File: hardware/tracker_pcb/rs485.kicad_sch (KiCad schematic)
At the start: 5 parts, among them IC3 THVD1426DRLR

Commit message: add opto input module
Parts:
- IC3: footprint SOTFL50P160X60-8N -> footprint:SOTFL50P160X60-8N
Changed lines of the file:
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@@
 			)
 		)
-		(property "Footprint" "SOTFL50P160X60-8N"
+		(property "Footprint" "footprint:SOTFL50P160X60-8N"
 			(at 144.78 169.85 0)
 			(effects

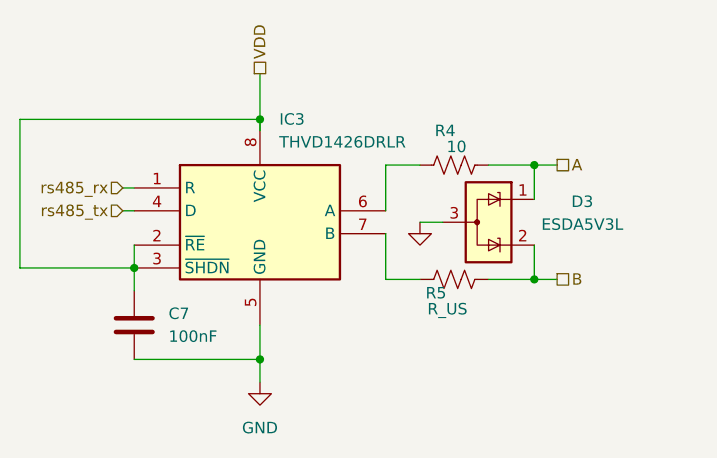
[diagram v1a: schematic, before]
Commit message: Work
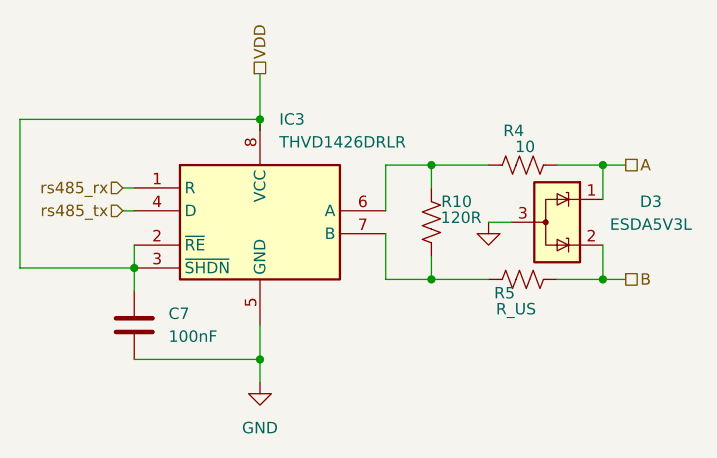
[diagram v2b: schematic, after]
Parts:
- added R10: 120R, Resistor_SMD:R_0603_1608Metric, symbol Device:R_US
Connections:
- net at IC3.6 (A), R4.1: now also R10.2
- net at IC3.7 (B), R5.1: now also R10.1
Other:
- moved on the sheet: D3, R4, R5
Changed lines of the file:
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@@
 	)
 	(junction
-		(at 165.1 72.39)
+		(at 172.72 72.39)
 		(diameter 0)
 		(color 0 0 0 0)
 	)
 	(junction
-		(at 165.1 85.09)
+		(at 172.72 85.09)
+		(diameter 0)
+		(color 0 0 0 0)
+	)
+	(junction
+		(at 153.67 72.39)
 		(diameter 0)
 		(color 0 0 0 0)
@@
 	)
 	(junction
+		(at 153.67 85.09)
+		(diameter 0)
+		(color 0 0 0 0)
+	)
+	(junction
 		(at 134.62 67.31)
 		(diameter 0)
@@
 	(wire
 		(pts
-			(xy 160.02 85.09) (xy 165.1 85.09)
+			(xy 167.64 85.09) (xy 172.72 85.09)
 		)
 		(stroke
@@
 	(wire
 		(pts
+			(xy 153.67 72.39) (xy 153.67 74.93)
+		)
+		(stroke
+			(width 0)
+			(type default)
+		)
+	)
+	(wire
+		(pts
 			(xy 134.62 93.98) (xy 134.62 96.52)
 		)
@@
 	(wire
 		(pts
-			(xy 165.1 72.39) (xy 165.1 76.2)
+			(xy 172.72 72.39) (xy 172.72 76.2)
 		)
 		(stroke
@@
 	(wire
 		(pts
-			(xy 160.02 72.39) (xy 165.1 72.39)
+			(xy 167.64 72.39) (xy 172.72 72.39)
+		)
+		(stroke
+			(width 0)
+			(type default)
+		)
+	)
+	(wire
+		(pts
+			(xy 153.67 72.39) (xy 160.02 72.39)
 		)
 		(stroke
@@
 	(wire
 		(pts
-			(xy 165.1 85.09) (xy 167.64 85.09)
+			(xy 153.67 82.55) (xy 153.67 85.09)
+		)
+		(stroke
+			(width 0)
+			(type default)
+		)
+	)
+	(wire
+		(pts
+			(xy 172.72 85.09) (xy 175.26 85.09)
 		)
 		(stroke
@@
 	(wire
 		(pts
+			(xy 153.67 85.09) (xy 160.02 85.09)
+		)
+		(stroke
+			(width 0)
+			(type default)
+		)
+	)
+	(wire
+		(pts
 			(xy 120.65 83.82) (xy 120.65 86.36)
 		)
@@
 	(wire
 		(pts
-			(xy 165.1 72.39) (xy 167.64 72.39)
-		)
-		(stroke
-			(width 0)
-			(type default)
-		)
-	)
-	(wire
-		(pts
-			(xy 152.4 78.74) (xy 154.94 78.74)
+			(xy 172.72 72.39) (xy 175.26 72.39)
+		)
+		(stroke
+			(width 0)
+			(type default)
+		)
+	)
+	(wire
+		(pts
+			(xy 160.02 78.74) (xy 162.56 78.74)
 		)
 		(stroke
@@
 	(wire
 		(pts
-			(xy 165.1 85.09) (xy 165.1 81.28)
+			(xy 172.72 85.09) (xy 172.72 81.28)
 		)
 		(stroke
@@
 	(wire
 		(pts
-			(xy 148.59 72.39) (xy 152.4 72.39)
-		)
-		(stroke
-			(width 0)
-			(type default)
-		)
-	)
-	(wire
-		(pts
-			(xy 148.59 85.09) (xy 152.4 85.09)
+			(xy 148.59 72.39) (xy 153.67 72.39)
+		)
+		(stroke
+			(width 0)
+			(type default)
+		)
+	)
+	(wire
+		(pts
+			(xy 148.59 85.09) (xy 153.67 85.09)
 		)
 		(stroke
@@
 	(hierarchical_label "B"
 		(shape passive)
-		(at 167.64 85.09 0)
+		(at 175.26 85.09 0)
 		(effects
 			(font
@@
 	(hierarchical_label "A"
 		(shape passive)
-		(at 167.64 72.39 0)
+		(at 175.26 72.39 0)
 		(effects
 			(font
@@
 	(symbol
 		(lib_id "Power_Protection:ESDA5V3L")
-		(at 160.02 78.74 270)
+		(at 167.64 78.74 270)
 		(unit 1)
 		(exclude_from_sim no)
@@
 		(dnp no)
 		(property "Reference" "D3"
-			(at 170.434 76.454 90)
+			(at 178.054 76.454 90)
 			(effects
 				(font
@@
 		)
 		(property "Value" "ESDA5V3L"
-			(at 170.434 78.994 90)
+			(at 178.054 78.994 90)
 			(effects
 				(font
@@
 		)
 		(property "Footprint" "Package_TO_SOT_SMD:SOT-23-3"
-			(at 149.86 63.5 0)
+			(at 157.48 63.5 0)
 			(effects
 				(font
@@
 		)
 		(property "Datasheet" "https://www.st.com/resource/en/datasheet/esdal.pdf"
-			(at 144.78 78.74 0)
+			(at 152.4 78.74 0)
 			(effects
 				(font
@@
 		)
 		(property "Description" "TVS Diode Array, 5.5V Standoff, 2 Channels, SOT23"
-			(at 147.32 78.74 0)
+			(at 154.94 78.74 0)
 			(effects
 				(font
@@
 	)
 	(symbol
+		(lib_id "Device:R_US")
+		(at 153.67 78.74 180)
+		(unit 1)
+		(exclude_from_sim no)
+		(in_bom yes)
+		(on_board yes)
+		(dnp no)
+		(property "Reference" "R10"
+			(at 156.464 76.454 0)
+			(effects
+				(font
+					(size 1.27 1.27)
+				)
+			)
+		)
+		(property "Value" "120R"
+			(at 156.972 78.232 0)
+			(effects
+				(font
+					(size 1.27 1.27)
+				)
+			)
+		)
+		(property "Footprint" "Resistor_SMD:R_0603_1608Metric"
+			(at 152.654 78.486 90)
+			(effects
+				(font
+					(size 1.27 1.27)
+				)
+				(hide yes)
+			)
+		)
+		(property "Datasheet" "~"
+			(at 153.67 78.74 0)
+			(effects
+				(font
+					(size 1.27 1.27)
+				)
+				(hide yes)
+			)
+		)
+		(property "Description" "Resistor, US symbol"
+			(at 153.67 78.74 0)
+			(effects
+				(font
+					(size 1.27 1.27)
+				)
+				(hide yes)
+			)
+		)
+		(pin "2"
+		)
+		(pin "1"
+		)
+		(instances
+			(project "tracker_pcb"
+				(path "/6aaa9514-f94e-4843-90d0-16960e4e49cb/503eaca2-35bd-4283-8689-99ba385163a1"
+					(reference "R10")
+					(unit 1)
+				)
+			)
+		)
+	)
+	(symbol
 		(lib_id "power:GND")
-		(at 152.4 78.74 0)
+		(at 160.02 78.74 0)
 		(unit 1)
 		(exclude_from_sim no)
@@
 		(fields_autoplaced yes)
 		(property "Reference" "#PWR07"
-			(at 152.4 85.09 0)
+			(at 160.02 85.09 0)
 			(effects
 				(font
@@
 		)
 		(property "Value" "GND"
-			(at 152.4 83.82 0)
+			(at 160.02 83.82 0)
 			(effects
 				(font
@@
 		)
 		(property "Footprint" ""
-			(at 152.4 78.74 0)
+			(at 160.02 78.74 0)
 			(effects
 				(font
@@
 		)
 		(property "Datasheet" ""
-			(at 152.4 78.74 0)
+			(at 160.02 78.74 0)
 			(effects
 				(font
@@
 		)
 		(property "Description" "Power symbol creates a global label with name \"GND\" , ground"
-			(at 152.4 78.74 0)
+			(at 160.02 78.74 0)
 			(effects
 				(font
@@
 	(symbol
 		(lib_id "Device:R_US")
-		(at 156.21 72.39 90)
+		(at 163.83 72.39 90)
 		(unit 1)
 		(exclude_from_sim no)
@@
 		(dnp no)
 		(property "Reference" "R4"
-			(at 155.194 68.58 90)
+			(at 162.814 68.58 90)
 			(effects
 				(font
@@
 		)
 		(property "Value" "10"
-			(at 156.464 70.358 90)
+			(at 164.084 70.358 90)
 			(effects
 				(font
@@
 		)
 		(property "Footprint" "Resistor_SMD:R_0603_1608Metric"
-			(at 156.464 71.374 90)
+			(at 164.084 71.374 90)
 			(effects
 				(font
@@
 		)
 		(property "Datasheet" "~"
-			(at 156.21 72.39 0)
+			(at 163.83 72.39 0)
 			(effects
 				(font
@@
 		)
 		(property "Description" "Resistor, US symbol"
-			(at 156.21 72.39 0)
+			(at 163.83 72.39 0)
 			(effects
 				(font
@@
 	(symbol
 		(lib_id "Device:R_US")
-		(at 156.21 85.09 90)
+		(at 163.83 85.09 90)
 		(unit 1)
 		(exclude_from_sim no)
@@
 		(dnp no)
 		(property "Reference" "R5"
-			(at 154.178 86.614 90)
+			(at 161.798 86.614 90)
 			(effects
 				(font
@@
 		)
 		(property "Value" "R_US"
-			(at 155.448 88.392 90)
+			(at 163.068 88.392 90)
 			(effects
 				(font
@@
 		)
 		(property "Footprint" "Resistor_SMD:R_0603_1608Metric"
-			(at 156.464 84.074 90)
+			(at 164.084 84.074 90)
 			(effects
 				(font
@@
 		)
 		(property "Datasheet" "~"
-			(at 156.21 85.09 0)
+			(at 163.83 85.09 0)
 			(effects
 				(font
@@
 		)
 		(property "Description" "Resistor, US symbol"
-			(at 156.21 85.09 0)
-			(effects
-				(font
+			(at 163.83 85.09 0)
+			(effects
+				(font
